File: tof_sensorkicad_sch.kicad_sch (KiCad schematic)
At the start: 1 part

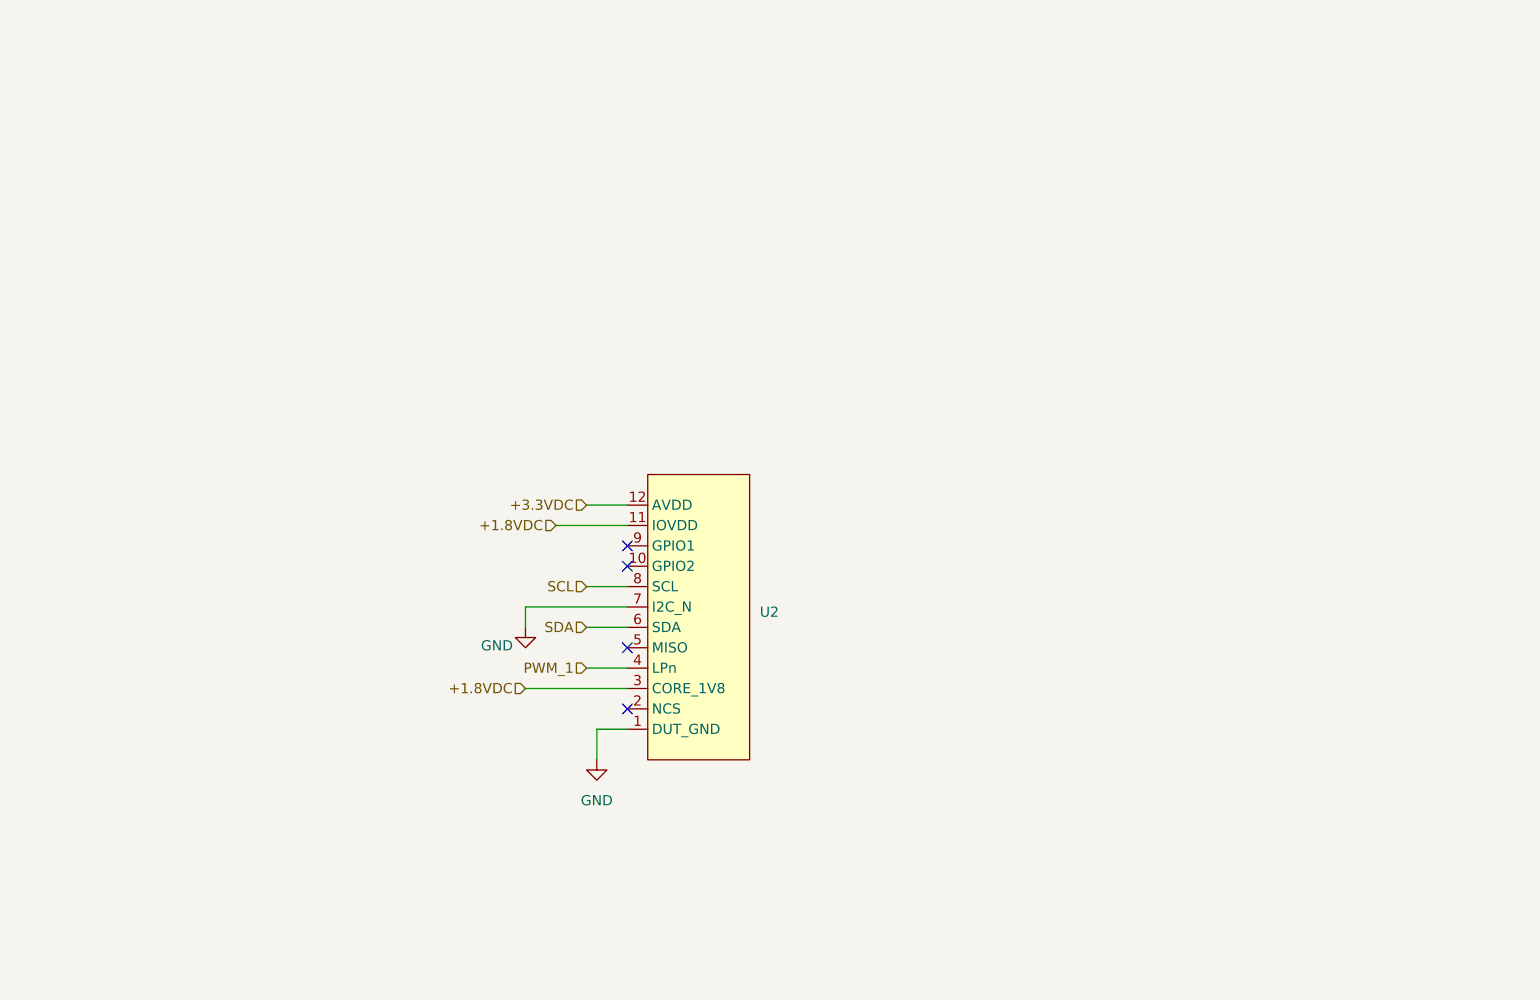
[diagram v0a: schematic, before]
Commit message: made board
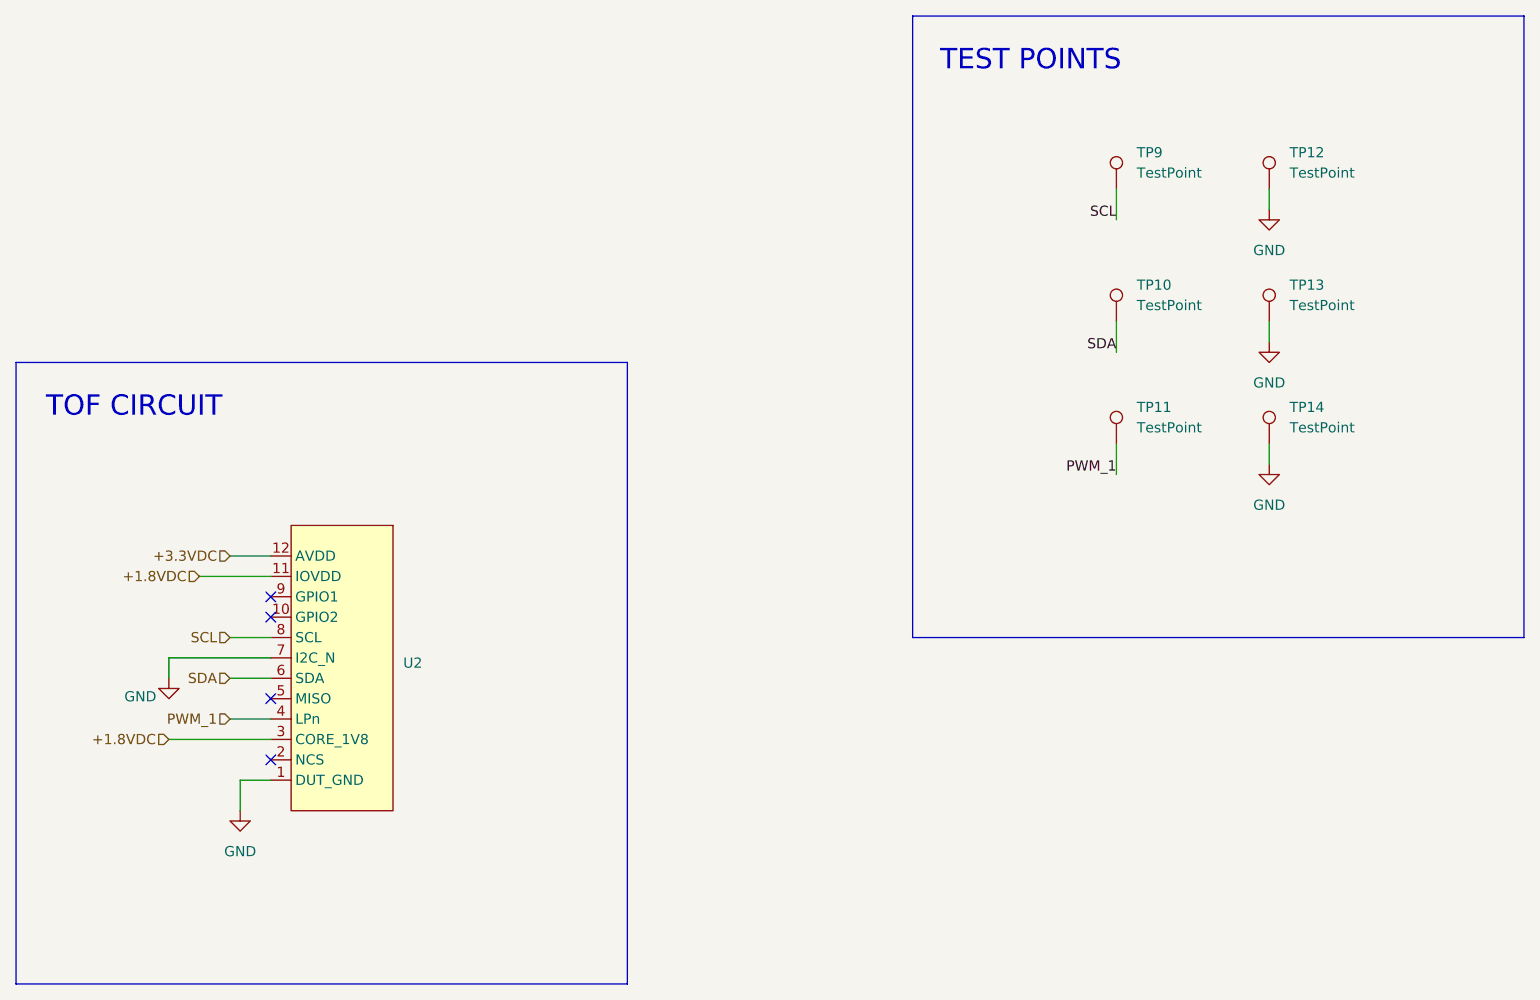
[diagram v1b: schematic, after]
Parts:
- added TP10, TP11, TP12, TP13, TP14, TP9: TestPoint, TestPoint:TestPoint_Pad_D2.0mm, symbol Connector:TestPoint
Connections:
- net GND: now also TP12.1, TP13.1, TP14.1
- net PWM_1: now also TP11.1
- net SCL: now also TP9.1
- net SDA: now also TP10.1
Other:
- note added: "TEST POINTS"
- note added: "TOF CIRCUIT"
- moved on the sheet: U2
